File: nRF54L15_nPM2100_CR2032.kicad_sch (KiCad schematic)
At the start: 50 parts, among them J1 Conn_ARM_SWD_TagConnect_TC203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, Q1 Q_NMOS_GSD, SW1 SW_Push, U1 nRF54L15-CAXX, U2 nPM2100-CAXX, U3 ADXL366, Y1 32.768kHz, Y2 SiT11100

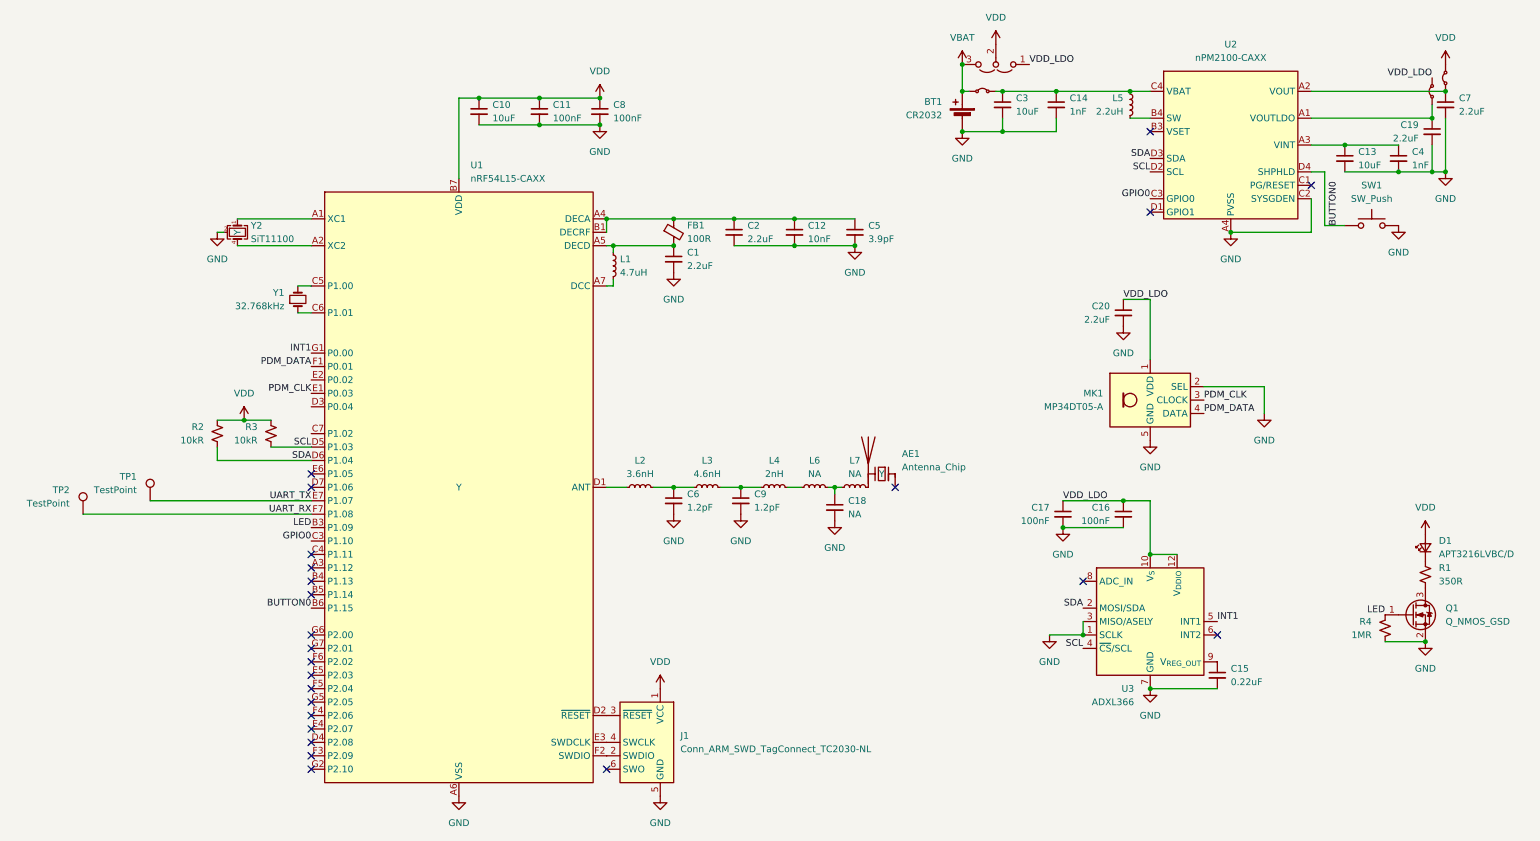
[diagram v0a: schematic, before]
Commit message: Dec92024
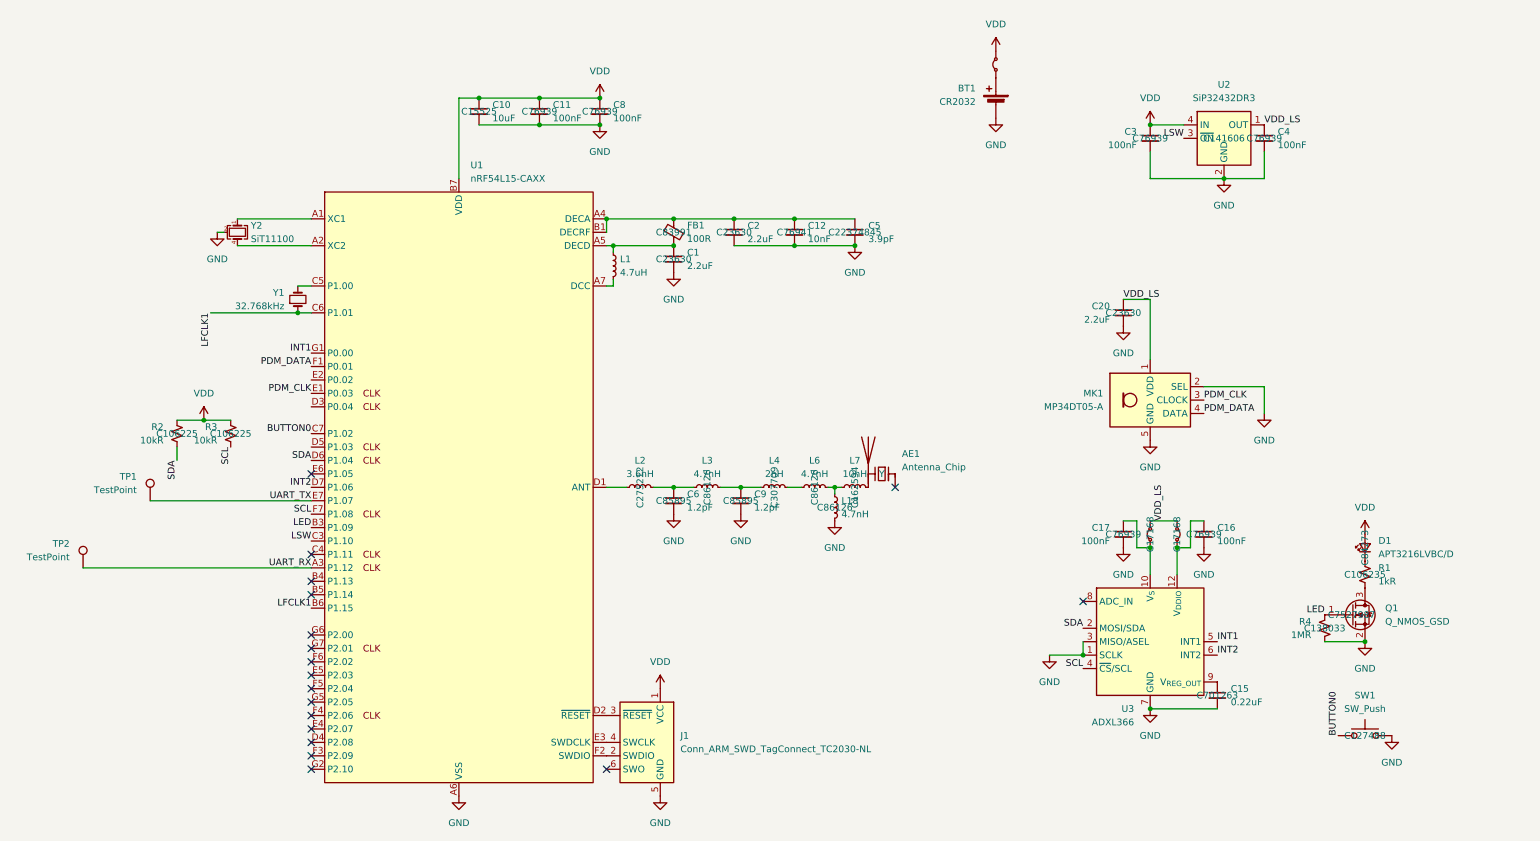
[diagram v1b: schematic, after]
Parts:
- removed C13: 10uF, Capacitor_SMD:C_0402_1005Metric, symbol Device:C_Small
- removed C14: 1nF, Capacitor_SMD:C_0201_0603Metric, symbol Device:C_Small
- removed C19, C7: 2.2uF, Capacitor_SMD:C_0201_0603Metric, symbol Device:C_Small
- removed JP2: Jumper_3_Open, Jumper:SolderJumper-3_P1.3mm_Open_RoundedPad1.0x1.5mm, symbol Jumper:Jumper_3_Open
- removed JP4: Jumper_2_Small_Bridged, Jumper:SolderJumper-2_P1.3mm_Bridged_RoundedPad1.0x1.5mm, symbol Jumper:Jumper_2_Small_Bridged
- removed L5: 2.2uH, Inductor_SMD:L_0402_1005Metric, symbol Device:L_Small
- removed U2: nPM2100-CAXX, nordic-lib-kicad-npm:BGA-16_4x4_1.9175x1.8975mm, symbol nordic-lib-kicad-npm:nPM2100-CAXX
- added JP2: Jumper_2_Small_Bridged, Resistor_SMD:R_0402_1005Metric, symbol Jumper:Jumper_2_Small_Bridged
- added U2: SiP32432DR3, Package_TO_SOT_SMD:SOT-363_SC-70-6, symbol Power_Management:SiP32432DR3
- C1, C2, C20: LCSC (none) -> C23630
- C10: LCSC (none) -> C15525
- C11, C16, C17, C8: LCSC (none) -> C76939
- C12: LCSC (none) -> C76941
- C15: LCSC (none) -> C701263
- C3: value 10uF -> 100nF; footprint Capacitor_SMD:C_0402_1005Metric -> Capacitor_SMD:C_0201_0603Metric; LCSC (none) -> C76939
- C4: value 1nF -> 100nF; LCSC (none) -> C76939
- C5: LCSC (none) -> C22374845
- C6, C9: LCSC (none) -> C85895
- D1: LCSC (none) -> C84273
- FB1: LCSC (none) -> C83991
- JP3: footprint Jumper:SolderJumper-2_P1.3mm_Bridged_RoundedPad1.0x1.5mm -> Resistor_SMD:R_0402_1005Metric; LCSC (none) -> C17168
- L18: renamed from C18; value NA -> 4.7nH; symbol Device:C_Small -> Device:L_Small; LCSC (none) -> C86126
- L2: LCSC (none) -> C275212
- L3: value 4.6nH -> 4.7nH; LCSC (none) -> C86126
- L4: LCSC (none) -> C307709
- L6: value NA -> 4.7nH; footprint Inductor_SMD:L_0201_0603Metric -> Capacitor_SMD:C_0201_0603Metric; LCSC (none) -> C86126
- L7: value NA -> 10nH; footprint Inductor_SMD:L_0201_0603Metric -> Capacitor_SMD:C_0201_0603Metric; LCSC (none) -> C162594
- Q1: LCSC (none) -> C7527987
- R1: value 350R -> 1kR; LCSC (none) -> C106235
- R2, R3: LCSC (none) -> C106225
- R4: LCSC (none) -> C138033
- SW1: LCSC (none) -> C127488
- U1: footprint nordic-lib-kicad-nrf54:BGA-49_7x7_2.3984x2.2309mm -> nordic-lib-kicad-nrf54:BGA-47_7x7_2.451x2.245mm
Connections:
- net BUTTON0: now also U1.C7 (P1.02); no longer U1.B6 (P1.15)
- net GND: now also U2.2 (GND), U2.5 (GND)
- net SCL: now also U1.F7 (P1.08); no longer U1.D5 (P1.03)
- net UART_RX: now also U1.A3 (P1.12); no longer U1.F7 (P1.08)
- net VDD: now also C3.1, JP1.2 (B), U2.4 (IN); no longer JP3.2 (B)
- net INT2: now reaches U3.6 (INT2)
- net INT2: now also U1.D7 (P1.06)
- net LFCLK1: now reaches U1.C6 (P1.01), Y1.1
- net LFCLK1: now also U1.B6 (P1.15)
- net at JP3.1 (A): now also C17.1, U3.10 (V_{S})
- net VDD_LS: now reaches C4.1
- net VDD_LS: now also C20.1, JP3.2 (B), MK1.1 (VDD), JP2.2 (B), U2.1 (OUT)
- net GPIO0 renamed LSW
- net LSW: now also U2.3 (~{ON})
- net VBAT: no longer names the net of BT1.1 (+), JP1.1 (A)
- removed net VDD_LDO: C16.1, C17.1, C20.1, MK1.1 (VDD), U3.10 (V_{S}), U3.12 (V_{DDIO})
- new net: C16.1, JP2.1 (A), U3.12 (V_{DDIO})
- no-connect marks 24 -> 18
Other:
- moved on the sheet: C15, C16, C17, D1, Q1, R1, R2, R3, R4, SW1, TP2, U3
